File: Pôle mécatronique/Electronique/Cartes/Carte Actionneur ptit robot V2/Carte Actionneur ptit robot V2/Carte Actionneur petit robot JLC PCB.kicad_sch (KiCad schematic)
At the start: 37 parts, among them Q1 BC557, U1 MCP2551-I-P

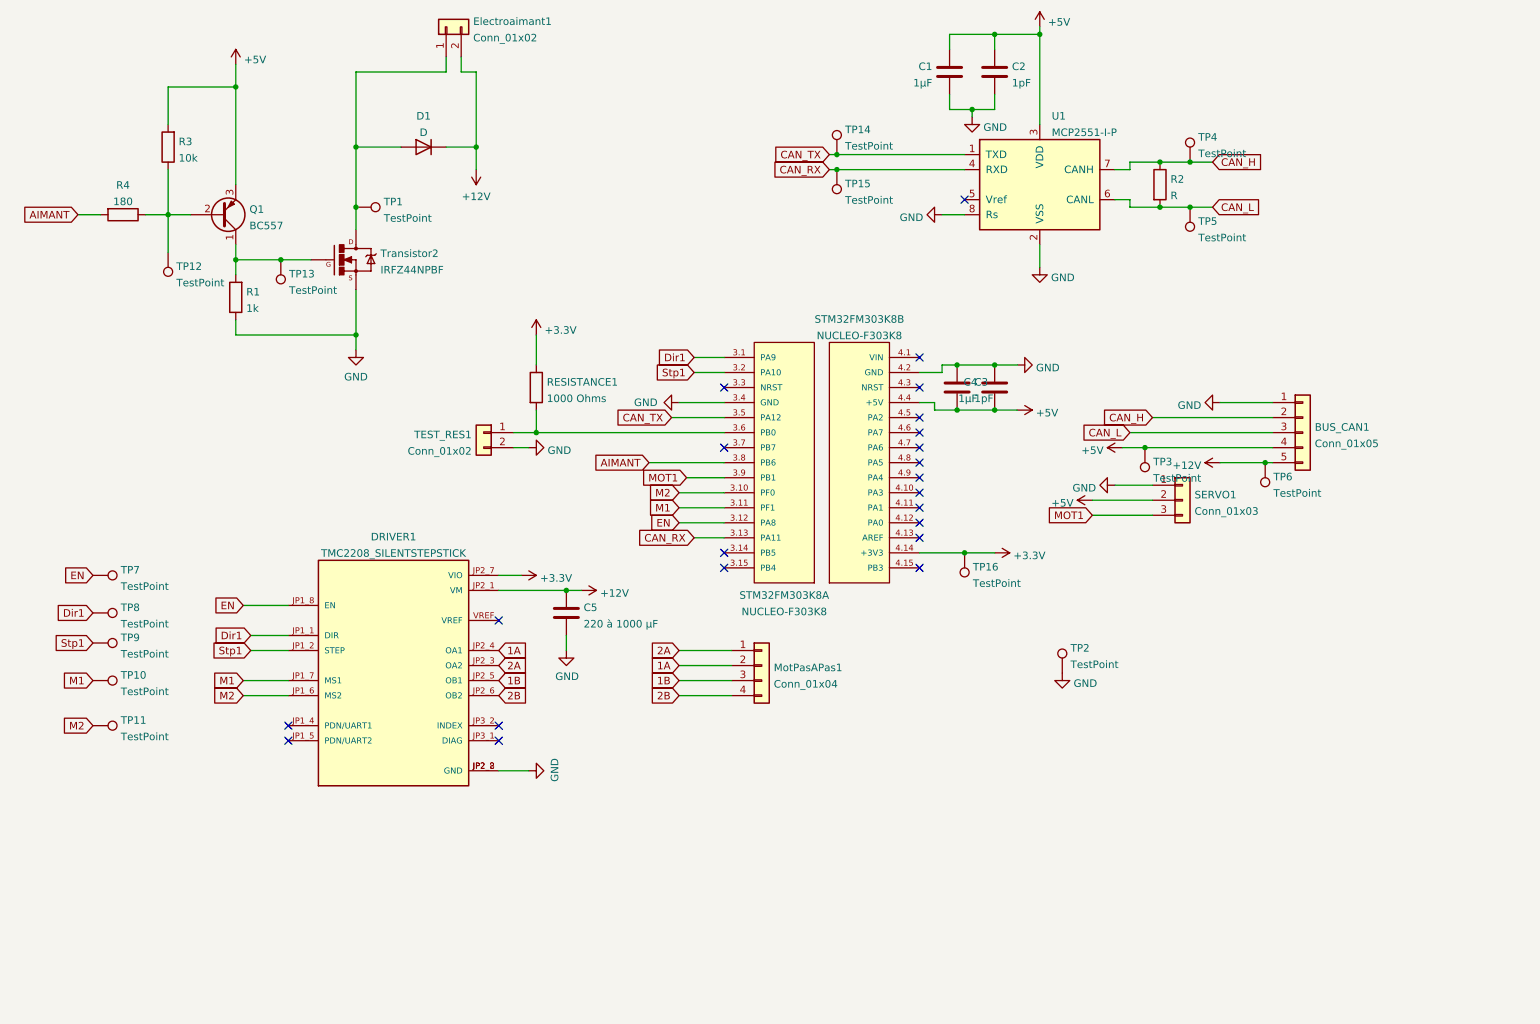
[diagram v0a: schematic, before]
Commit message: Up random
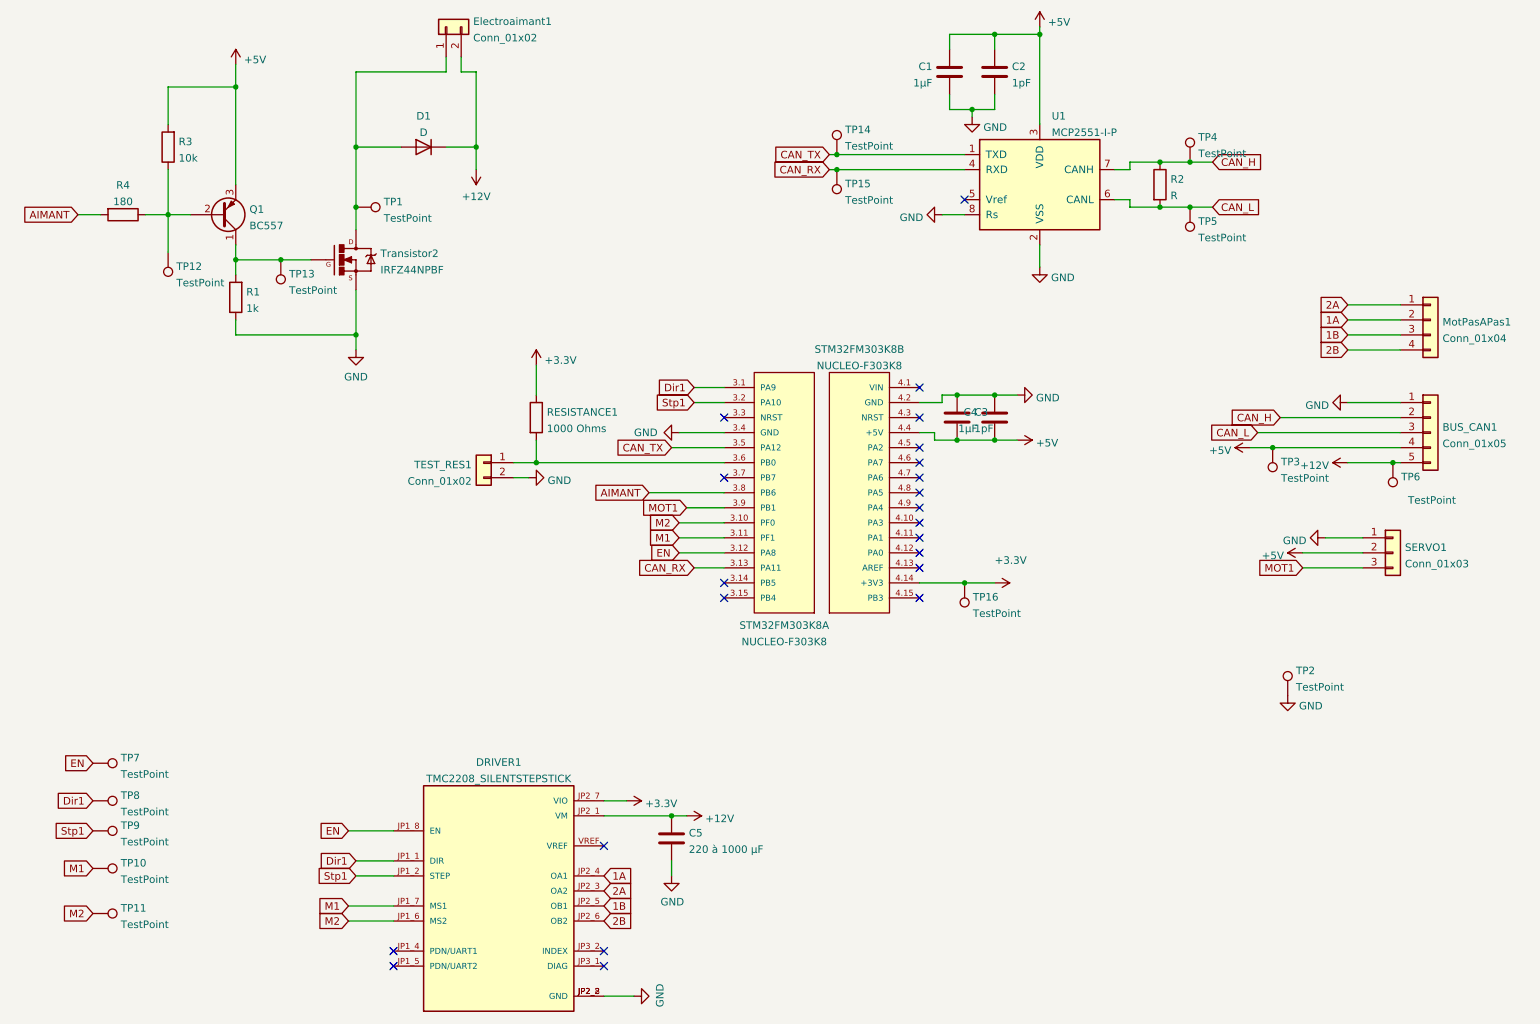
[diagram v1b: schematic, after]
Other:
- moved on the sheet: BUS_CAN1, C3, C4, C5, DRIVER1, MotPasAPas1, RESISTANCE1, SERVO1, STM32FM303K8A, STM32FM303K8B, TEST_RES1, TP10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
